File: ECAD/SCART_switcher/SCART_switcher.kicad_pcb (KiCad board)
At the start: 4 copper layers, 262 x 125 mm, 82 parts, among them J1 SCART-F, Q1 BC847, Q2 BC847, Q24 BC847, Q25 BC847, Q26 2SK209, Q27 2SK209, U137 74LVC1G14, U2 74LVC1G08, U34 74LVC1G08, U35 CD4066, U36 74LVC1G04, U37 74LVC1G08, U38 74LVC1G08, U60 74LVC1G3157, U61 74LVC1G3157, U62 74LVC1G3157, U63 74LVC1G3157, U64 74LVC1G3157

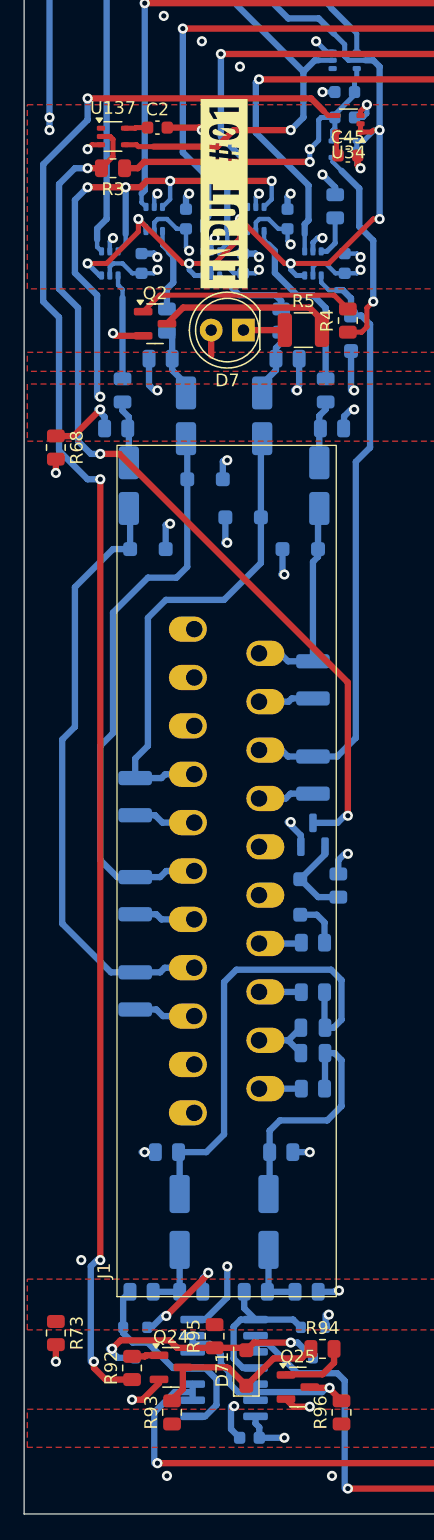
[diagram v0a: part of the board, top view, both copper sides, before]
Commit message: Update SCART_switcher.kicad_pcb
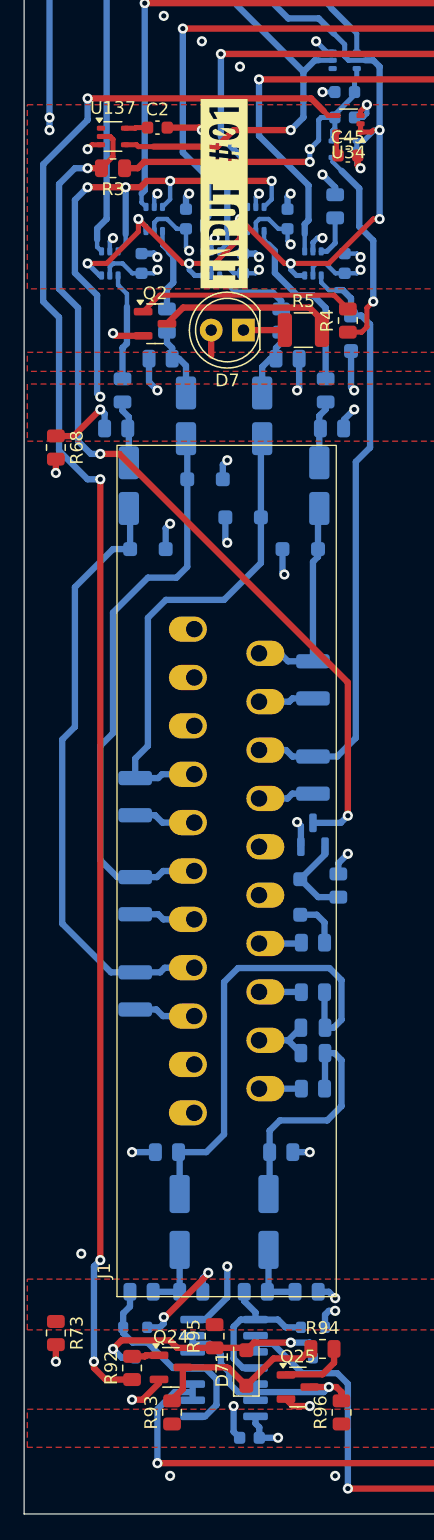
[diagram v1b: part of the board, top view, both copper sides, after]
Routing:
- net GND: track 98.4 -> 96.4 mm
- net +4V5: track 10.5 -> 12.1 mm
- net /SCART input 1/Audio input stage/AUDIO_OUT_ENABLE: track 18.7 -> 19.3 mm
- net Net-(Q1-C): track 70.5 -> 71.0 mm
